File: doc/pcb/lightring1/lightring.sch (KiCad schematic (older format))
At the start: 114 parts, among them J1 Conn_01x05_Female, J2 USB_B_Micro, J3 plate, SW2 SW_SPST, U1 STM32G070RBT, U2 MCP73831-2-OT, U3 AT42QT1012-T, U4 LDK130-33_SOT23_SOT353, Y1 Crystal

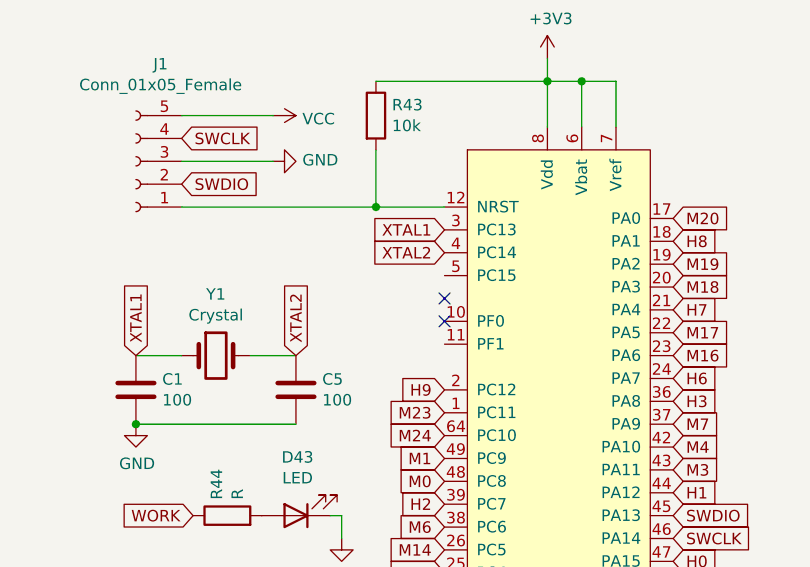
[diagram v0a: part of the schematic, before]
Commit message: initial program
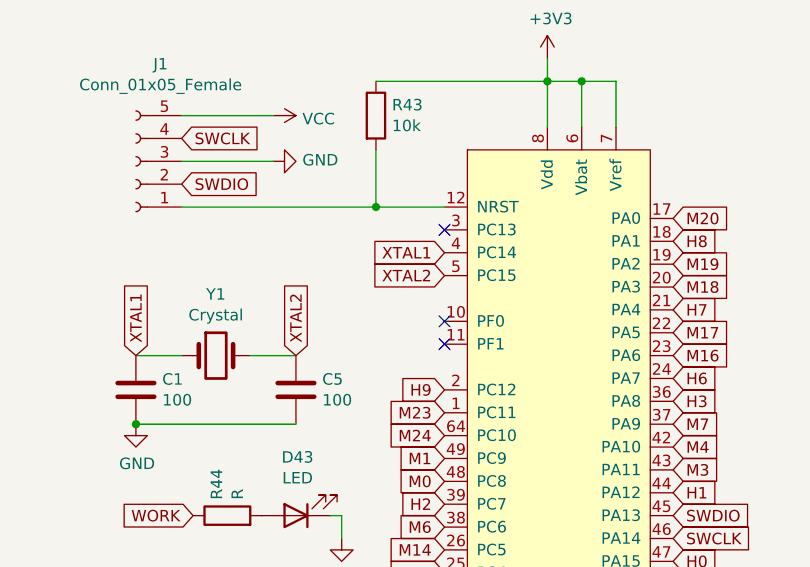
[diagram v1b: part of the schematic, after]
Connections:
- net XTAL1: now also U1.4 (PC14); no longer U1.3 (PC13)
- net XTAL2: now also U1.5 (PC15); no longer U1.4 (PC14)
- no-connect marks 14 -> 15
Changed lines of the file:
@@
 Wire Wire Line
 	9200 2700 9500 2700
-Text GLabel 9500 2800 0    50   Input ~ 0
+Text GLabel 9500 2900 0    50   Input ~ 0
 XTAL1
-Text GLabel 9500 2900 0    50   Input ~ 0
+Text GLabel 9500 3000 0    50   Input ~ 0
 XTAL2
 Text GLabel 9500 5100 0    50   Input ~ 0
@@
 WORK
 NoConn ~ 9500 4700
+NoConn ~ 9500 3300
 NoConn ~ 9500 3200
-NoConn ~ 9500 3100
 $Comp
 L Device:R R44
@@
 Text GLabel 9500 4600 0    50   Input ~ 0
 TOUCH
+NoConn ~ 9500 2800
 $EndSCHEMATC
